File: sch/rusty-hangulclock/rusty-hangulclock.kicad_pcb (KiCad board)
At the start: 2 copper layers, 53.5 x 54 mm, 13 parts, among them J1 Conn_OLED, J2 Conn_LEDS, J3 PWR, SW1 SW_Push

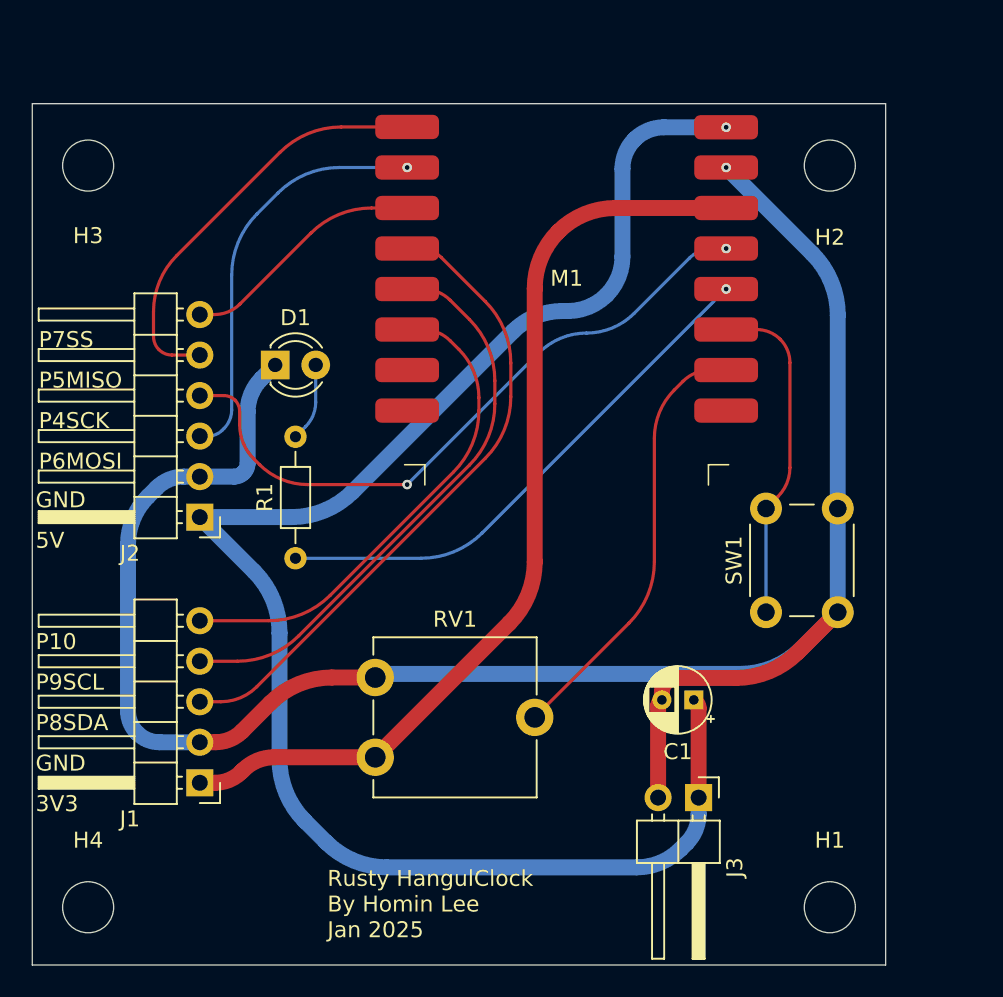
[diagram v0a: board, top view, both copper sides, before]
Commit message: fix sch and pcb
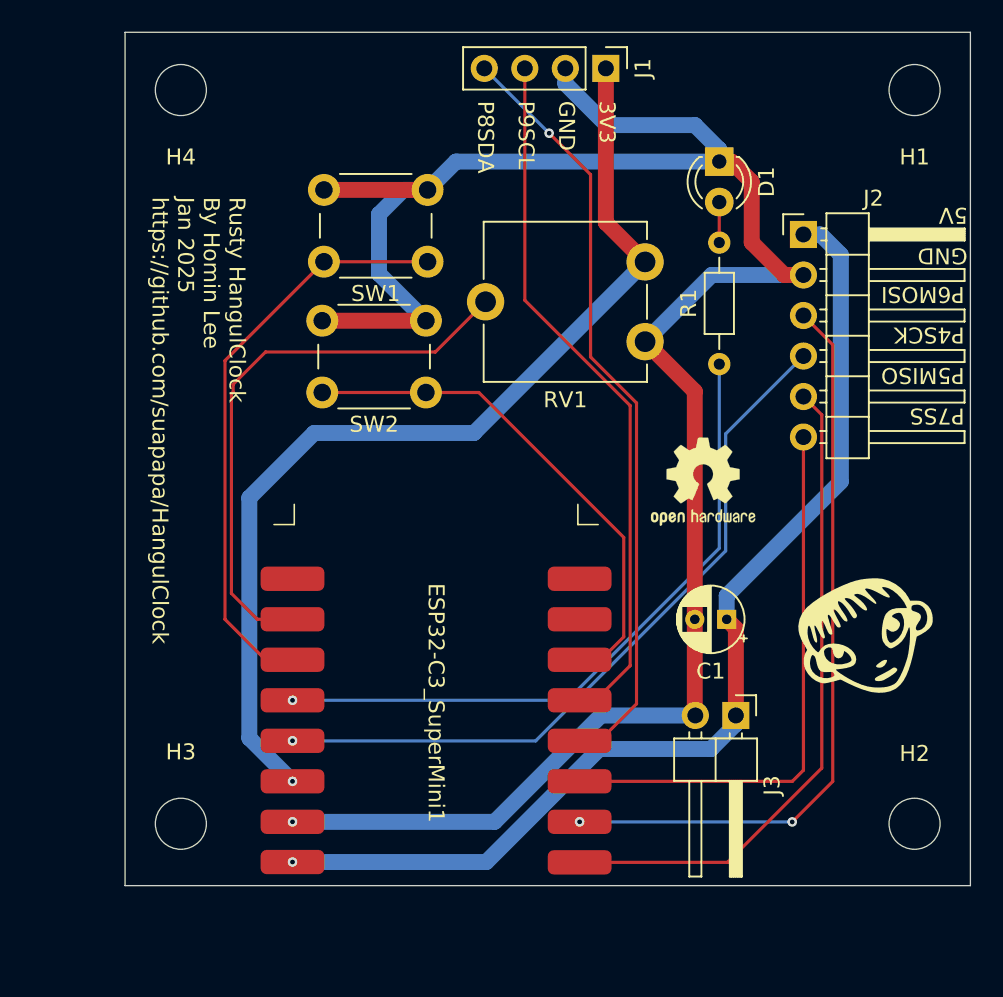
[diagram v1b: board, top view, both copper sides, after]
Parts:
- added G***: LOGO, LOGO, F.Cu at (168.2, 114.0)
- added REF**: OSHW-Logo2_7.3x6mm_SilkScreen, Symbol:OSHW-Logo2_7.3x6mm_SilkScreen, F.Cu at (158.1, 104.3)
- added SW2: SW_Push, Button_Switch_THT:SW_PUSH_6mm, F.Cu at (140.7, 98.7)
- J1: footprint Connector_PinHeader_2.54mm:PinHeader_1x05_P2.54mm_Horizontal -> Connector_PinHeader_2.54mm:PinHeader_1x04_P2.54mm_Vertical
- moved H1 72.9 mm to (171.3, 79.8), turned to 180 degrees
- moved H2 66.2 mm to (171.3, 125.8), turned to 180 degrees
- moved H4 65.4 mm to (125.3, 79.8), turned to 180 degrees
- moved H3 57.9 mm to (125.3, 125.8), turned to 180 degrees
- moved J1 51.5 mm to (152.0, 78.4), turned to -90 degrees
- moved J2 41.8 mm to (164.3, 88.8), turned to 0 degrees
- moved RV1 35.4 mm to (154.4, 90.5), turned to 180 degrees
- moved D1 30.6 mm to (159.1, 84.2), turned to -90 degrees
- moved SW1 30.5 mm to (140.8, 90.5), turned to 180 degrees
- moved R1 29.2 mm to (159.1, 96.9)
- moved ESP32-C3_SuperMini1 27.4 mm to (141.3, 118.2), turned to 180 degrees
- moved J3 5.65 mm to (160.1, 119.0)
- moved C1 5.45 mm to (159.5, 113.0)
- renumbered M1 to ESP32-C3_SuperMini1, H4 to H1, H3 to H2, H2 to H3, H1 to H4
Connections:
- ESP32-C3_SuperMini1 pad 10: Net-(J1-Pin_5) -> Net-(ESP32-C3_SuperMini1-P10)
- ESP32-C3_SuperMini1 pad 8: Net-(J1-Pin_3) -> Net-(ESP32-C3_SuperMini1-P8)
- ESP32-C3_SuperMini1 pad 9: Net-(J1-Pin_4) -> Net-(ESP32-C3_SuperMini1-P9)
- J1 pad 3: Net-(J1-Pin_3) -> Net-(ESP32-C3_SuperMini1-P9)
- J1 pad 4: Net-(J1-Pin_4) -> Net-(ESP32-C3_SuperMini1-P8)
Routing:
- net Net-(ESP32-C3_SuperMini1-P8): track 0.00 -> 48.3 mm, vias 0 -> 1
- net Net-(ESP32-C3_SuperMini1-P9): track 0.00 -> 44.3 mm
- net Net-(J1-Pin_3): track 40.9 -> 0.00 mm
- net Net-(J1-Pin_4): track 36.2 -> 0.00 mm
- net +5V: track 102.6 -> 66.9 mm
- net Net-(ESP32-C3_SuperMini1-P10): track 0.00 -> 32.3 mm
- net Net-(J1-Pin_5): track 31.6 -> 0.00 mm
- net Net-(ESP32-C3_SuperMini1-P6): track 26.0 -> 46.9 mm, vias 1 -> 2
- net Net-(ESP32-C3_SuperMini1-P7): track 15.4 -> 35.2 mm
- net Net-(ESP32-C3_SuperMini1-P2): track 21.3 -> 37.8 mm
- net Net-(ESP32-C3_SuperMini1-P5): track 26.5 -> 41.4 mm
- net Net-(ESP32-C3_SuperMini1-P1): track 27.3 -> 36.6 mm
- net Net-(ESP32-C3_SuperMini1-P3): track 33.7 -> 42.2 mm
- net GND: track 126.1 -> 131.5 mm
- net Net-(ESP32-C3_SuperMini1-P4): track 42.0 -> 46.3 mm, vias 2 -> 1
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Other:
- board size 53.5 x 54 mm -> 53 x 53.5 mm
- board text added: "Rusty HangulClock By Homin Lee Jan 2025 https://github.com/suapapa/HangulClock"
- board text removed: "P10"
- board text removed: "Rusty HangulClock By Homin Lee Jan 2025"
